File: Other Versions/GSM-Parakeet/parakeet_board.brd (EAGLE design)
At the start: 35 x 38.5 mm, 14 parts, among them IC1 TP4056

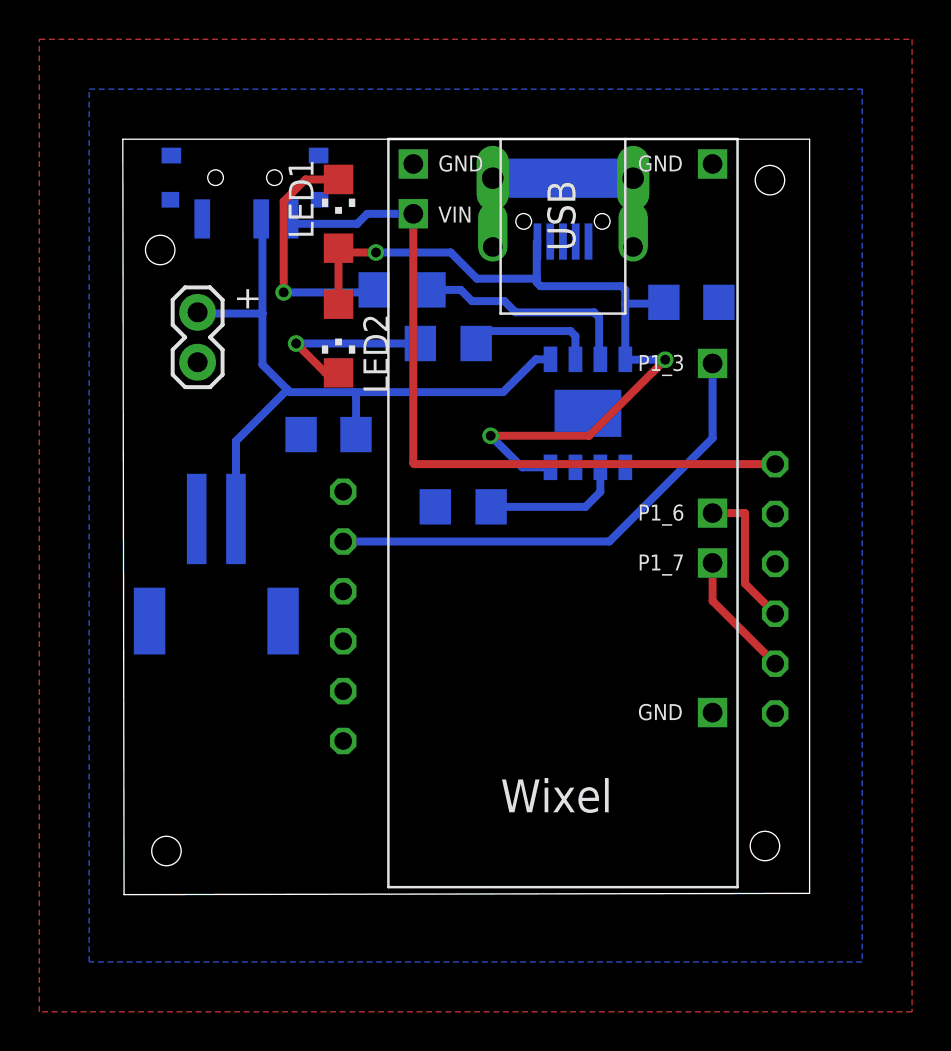
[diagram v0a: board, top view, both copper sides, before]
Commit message: Updated GSM version
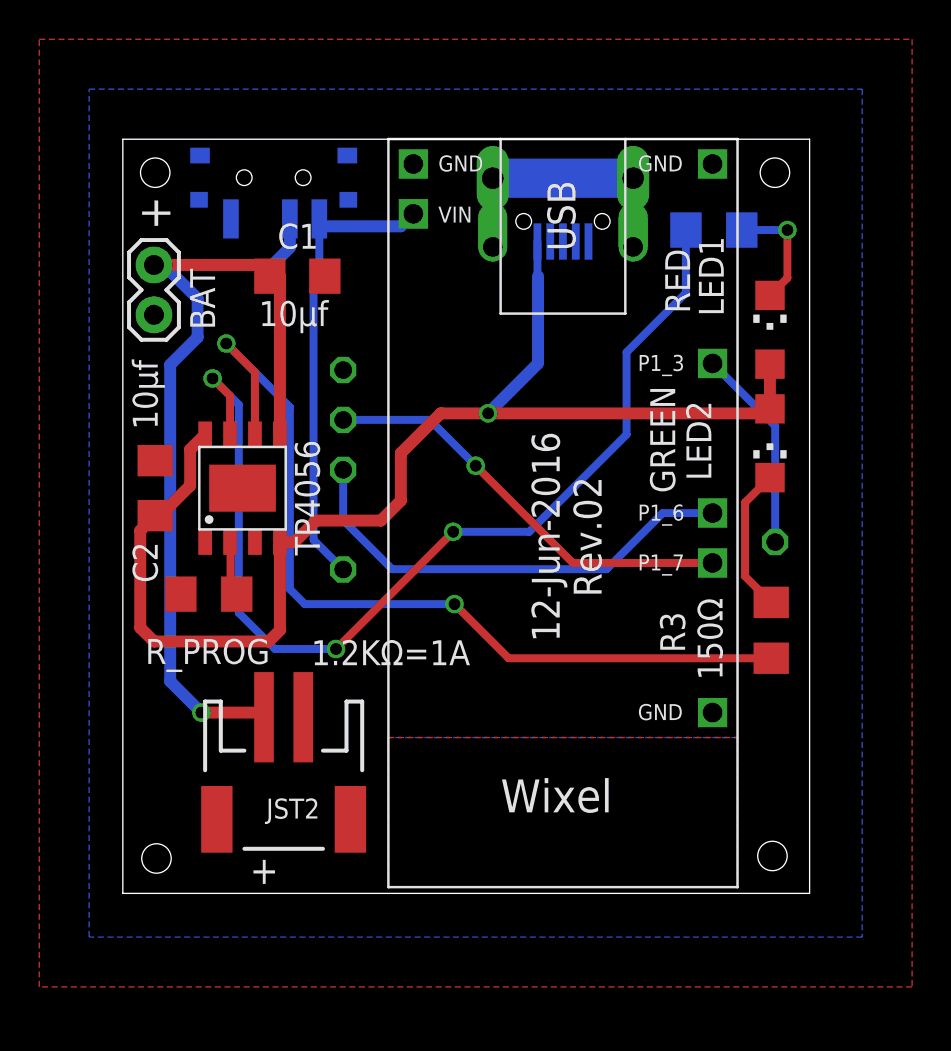
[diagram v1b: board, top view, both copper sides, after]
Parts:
- removed IC1: TP4056, TP4056:SOP-8
- removed U$2: SIM800L_GSM_MODULE, SIM800L Module:SIM800L_GSM_MODULE
- removed U$3: MSK-12C02_SMD_SPDT_SWITCH, MSK-12C02 SMD Micro Slider Switch SPDT:MSK-12C02
- added SIM800L: SIM800L_PARAKEET_ONLY, SIM800L Module:SIM800L_PARAKEET_ONLY
- added SWITCH: MSK-12C02_SMD_SPDT_SWITCH, MSK-12C02 SMD Micro Slider Switch SPDT:MSK-12C02
- added TP4056: TP4056, TP4056:SOP-8
- added USB: MICRO-USB-B, micro usb B - sparkfun - china - hole 4LEGS TEST:MICRO_USB_4_LEGS
- C1, C2: value 10uf -> 10μf
- R2, R3: value 1K -> 150Ω
- R_PROG: value 1.2K=1A -> 1.2KΩ=1A
- U$1: value MICRO-USB-B -> (none); device micro usb B - sparkfun - china - hole 4LEGS TEST:MICRO_USB_4_LEGS -> LOGO:PARAKEET_VECTOR
- moved C2 28.9 mm to (2.10, 62.2), flipped to the top, turned to 90 degrees
- moved U$1 27.2 mm to (8.89, 54.6), turned to 0 degrees
- moved LED1 22.8 mm to (33.4, 70.3)
- moved LED2 22.6 mm to (33.4, 64.5)
- moved R3 22.0 mm to (33.5, 55.0), flipped to the top, turned to 90 degrees
- moved R2 16.2 mm to (30.5, 75.4), turned to 180 degrees
- moved R_PROG 13.7 mm to (4.83, 56.8), flipped to the top, turned to 0 degrees
- moved JST2 10.7 mm to (8.64, 46.9), flipped to the top
- moved C1 8.22 mm to (9.33, 73.0), flipped to the top
- moved + 3.28 mm to (2.03, 73.6)
- renumbered U$4 to WIXEL
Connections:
- net GND: now also SIM800L.P$6_GND, TP4056.1, TP4056.3, USB.GND; no longer IC1.1, IC1.3, U$1.GND, U$2.P$6_GND
- net N$1: now also TP4056.2; no longer IC1.2
- net N$12: now also SIM800L.P$2_VIN, SWITCH.L1; no longer U$2.P$1, U$3.L1
- net N$13: now also SIM800L.P$8_DTR; no longer U$2.P$8_DTR
- net N$2: now also SIM800L.P$5_TXD; no longer U$2.P$5_TXD
- net N$5: now also TP4056.7; no longer IC1.7
- net N$6: now also TP4056.6; no longer IC1.6
- net N$7: now also TP4056.4, TP4056.8, USB.VCC; no longer IC1.4, IC1.8, U$1.VCC
- net N$8: now also SWITCH.COM, TP4056.5; no longer IC1.5, U$3.COM
- net N$9: now also SIM800L.P$4_RXD; no longer U$2.P$4_RXD
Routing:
- net N$5: track 11.4 -> 52.4 mm, vias 0 -> 3
- net N$6: track 6.61 -> 45.0 mm, vias 0 -> 2
- net N$7: track 42.2 -> 64.9 mm, vias 3 -> 1
- net N$9: track 7.41 -> 23.6 mm
- net N$2: track 6.45 -> 21.8 mm, vias 0 -> 1
- net N$8: track 36.6 -> 52.0 mm, vias 0 -> 1
- net N$13: track 24.8 -> 10.4 mm
- net N$12: track 37.7 -> 23.8 mm
- net N$3: track 12.6 -> 6.02 mm
- net N$1: track 7.13 -> 3.32 mm
- net N$4: track 9.10 -> 8.15 mm, vias 1 -> 0
- added copper zone on layer 16, net N$10
- added copper zone on layer 1, net N$11
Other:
- board size 35 x 38.5 mm -> 35 x 38.4 mm
- board text added: "12-Jun-2016 Rev.02"
